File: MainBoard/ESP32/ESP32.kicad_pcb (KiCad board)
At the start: 2 copper layers, 97.5 x 77 mm, 42 parts, among them J1 Ultrasonic_1, J10 OUT1, J11 OUT1, J12 OUT1, J13 OUT1, J14 OUT1, J15 OUT1, J16 pH_SNS, J17 TDS_SNS, J18 Temp_SNS, J2 Ultrasonic_2, J3 Ultrasonic_3, J4 Barrel_Jack_Switch, J5 USB_B, J6 I2C_1, J7 I2C_1, J8 I2C_1, J9 SD_CARD_Module, Q1 2N7000, Q2 2N7000, Q3 2N7000, Q4 2N7000, Q5 2N7000, U1 ATtiny85-20PU, U2 LM296, U3 AMS1117-3.3, U4 ESP32-DevKit_V1

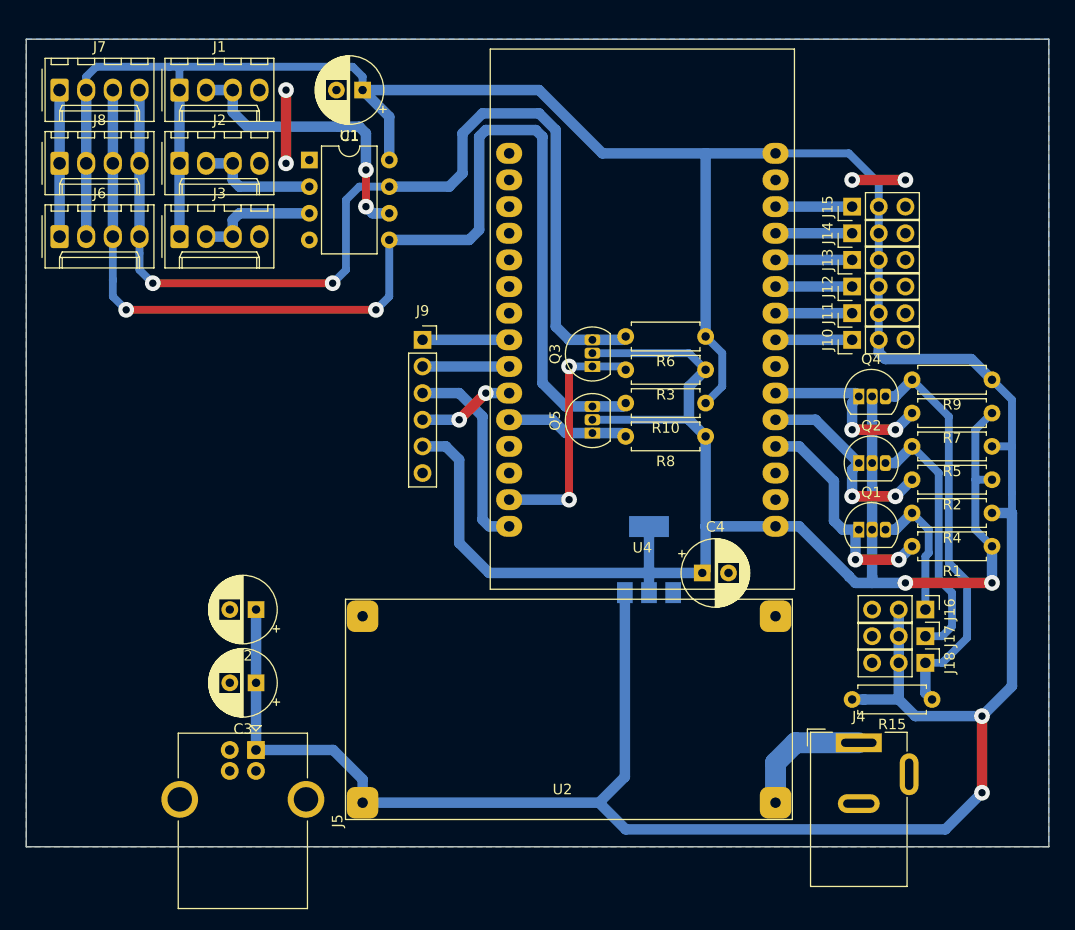
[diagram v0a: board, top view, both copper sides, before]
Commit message: Fix Main Board
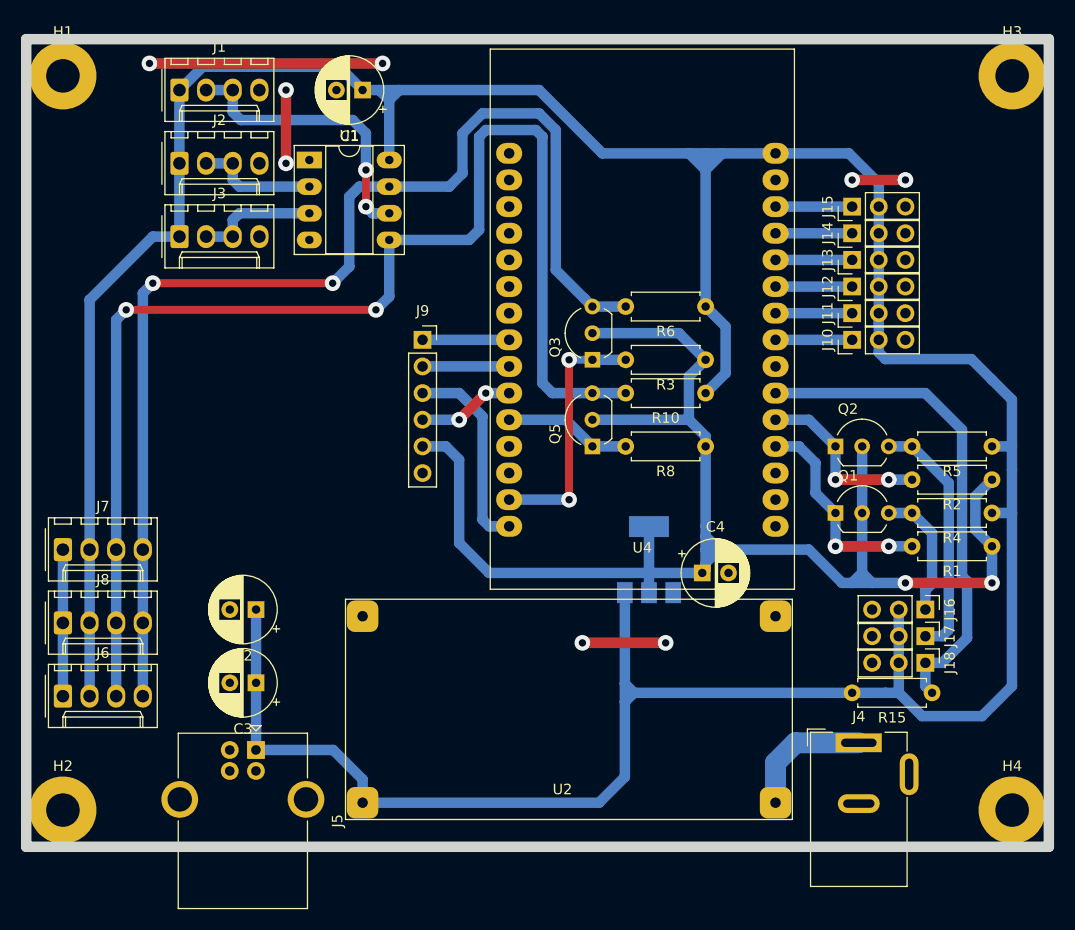
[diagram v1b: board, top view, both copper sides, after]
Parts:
- removed Q4: 2N7000, Package_TO_SOT_THT:TO-92L_Inline
- removed R7, R9: 10k, Resistor_THT:R_Axial_DIN0207_L6.3mm_D2.5mm_P7.62mm_Horizontal
- added H1: Mounting, MountingHole:MountingHole_3.2mm_M3_Pad, F.Cu at (107.0, 25.0)
- added H2: Mounting, MountingHole:MountingHole_3.2mm_M3_Pad, F.Cu at (107.0, 95.0)
- added H3: Mounting, MountingHole:MountingHole_3.2mm_M3_Pad, F.Cu at (197.5, 25.0)
- added H4: Mounting, MountingHole:MountingHole_3.2mm_M3_Pad, F.Cu at (197.5, 95.0)
- Q1, Q2, Q3, Q5: footprint Package_TO_SOT_THT:TO-92L_Inline -> Package_TO_SOT_THT:TO-92_Inline_Wide
- U1: footprint Package_DIP:DIP-8_W7.62mm -> Package_DIP:DIP-8_W7.62mm_Socket_LongPads
- moved J6 43.8 mm to (107.0, 84.1)
- moved J7 43.8 mm to (107.0, 70.2)
- moved J8 43.8 mm to (107.0, 77.2)
- moved R6 2.86 mm to (168.3, 47.0)
- moved Q1 2.73 mm to (180.7, 66.7)
- moved Q2 2.73 mm to (180.7, 60.3)
- moved Q5 1.27 mm to (157.5, 60.3)
- moved R10 0.95 mm to (168.3, 55.2)
- moved R3 0.95 mm to (168.3, 52.1)
- moved R8 0.95 mm to (168.3, 60.3)
- moved R15 0.64 mm to (189.9, 83.8)
- moved Q3 0.63 mm to (157.5, 52.1)
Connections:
- J18 pad 1: /H_TEMP_SNS -> /TEMP_SNS
- R15 pad 1: /H_TEMP_SNS -> /TEMP_SNS
- U4 pad 1: +3V3 -> Net-(U4-Pad1)
- U4 pad 6: /L_TEMP_SNS -> /TEMP_SNS
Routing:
- net /TEMP_SNS: track 0.00 -> 47.4 mm
- net /H_TEMP_SNS: track 38.7 -> 0.00 mm
- net GND: track 26.0 -> 56.2 mm, vias 4 -> 8
- net +5V: track 349.9 -> 379.0 mm, vias 2 -> 0
- net /L_TEMP_SNS: track 17.9 -> 0.00 mm, vias 2 -> 0
- net /H_SCL: track 96.9 -> 113.1 mm
- net /H_SDA: track 109.4 -> 124.5 mm
- net +3V3: track 150.5 -> 143.6 mm
- net /L_TDS_SNS: track 19.5 -> 17.2 mm
- net /L_pH_SNS: track 22.1 -> 20.5 mm
- net /H_TDS_SNS: track 24.9 -> 23.6 mm
- net /H_pH_SNS: track 13.2 -> 12.5 mm

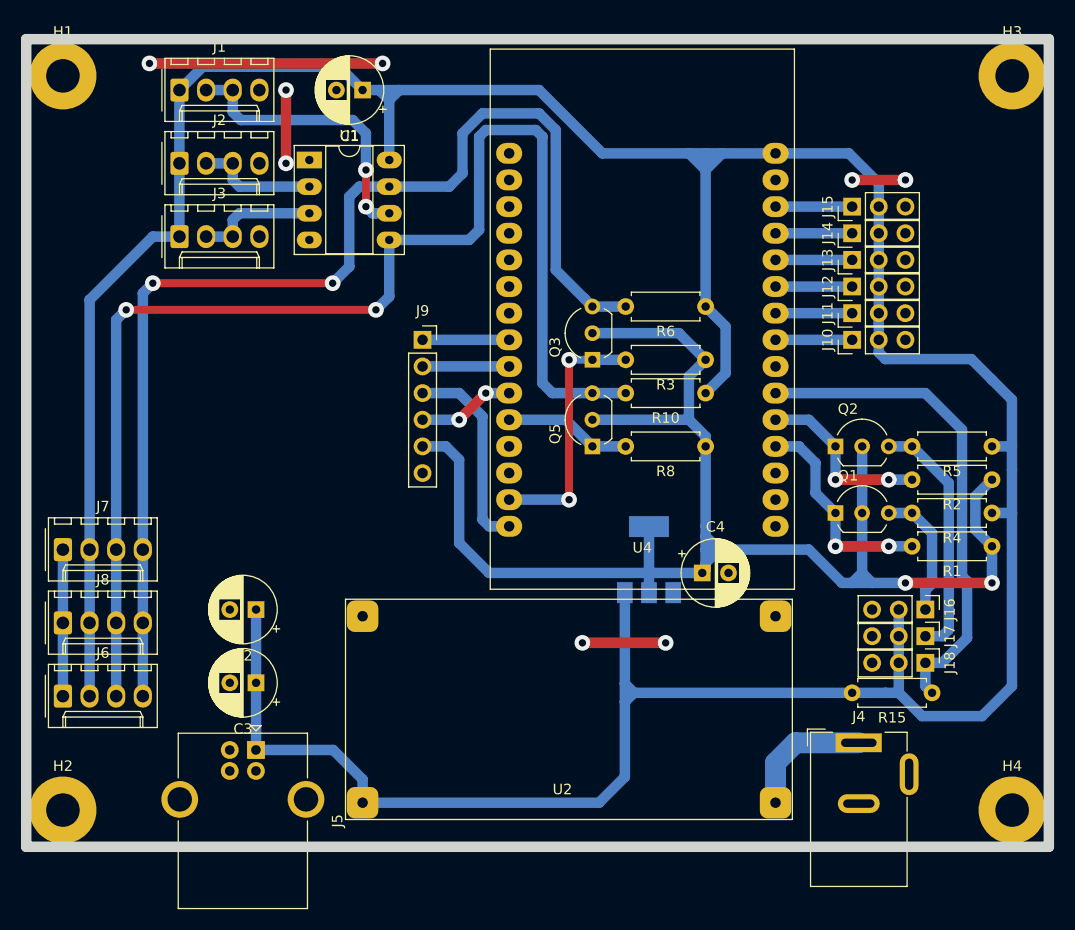
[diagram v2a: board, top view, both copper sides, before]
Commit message: Update Main Board
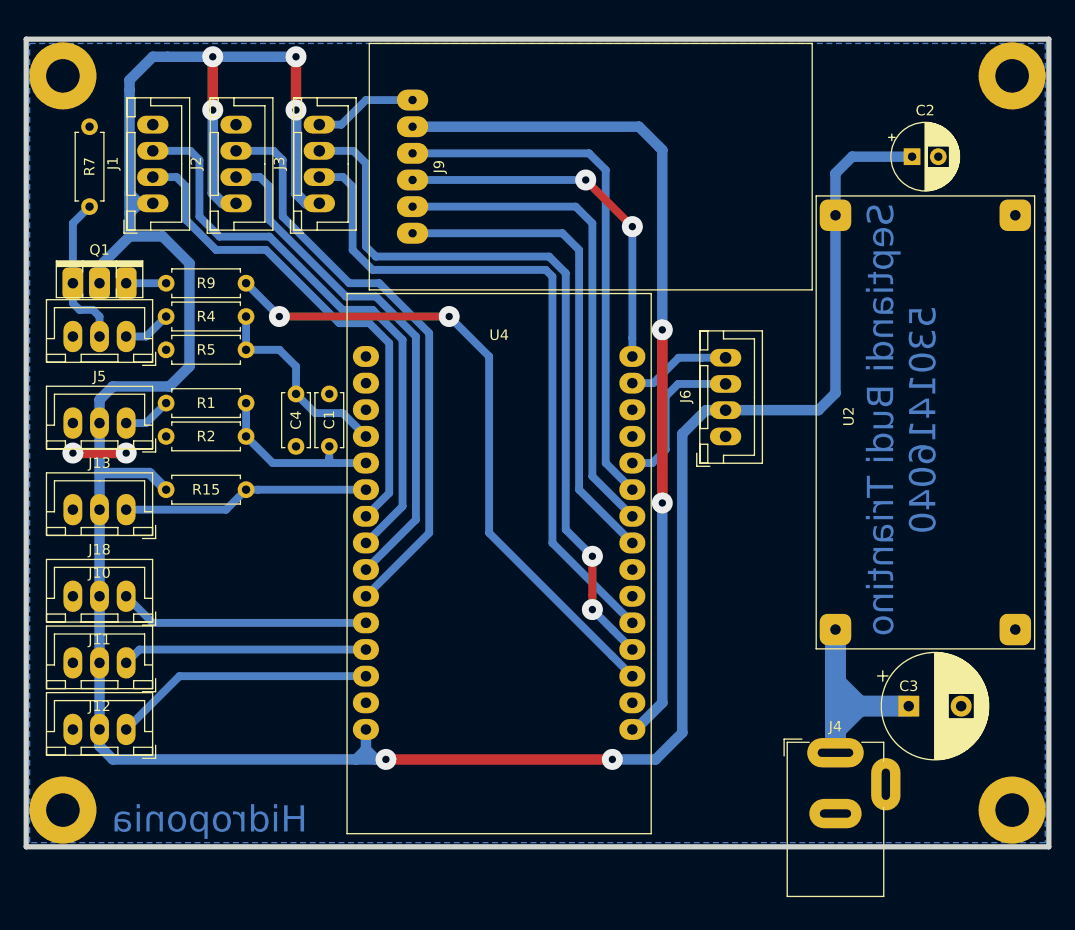
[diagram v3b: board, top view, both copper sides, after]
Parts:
- removed J14, J15: OUT1, Connector_PinHeader_2.54mm:PinHeader_1x03_P2.54mm_Vertical
- removed J16: pH_SNS, Connector_PinHeader_2.54mm:PinHeader_1x03_P2.54mm_Vertical
- removed J17: TDS_SNS, Connector_PinHeader_2.54mm:PinHeader_1x03_P2.54mm_Vertical
- removed J7, J8: I2C_1, Connector_Molex:Molex_KK-254_AE-6410-04A_1x04_P2.54mm_Vertical
- removed Q2, Q3, Q5: 2N7000, Package_TO_SOT_THT:TO-92_Inline_Wide
- removed R10, R3, R6, R8: 10k, Resistor_THT:R_Axial_DIN0207_L6.3mm_D2.5mm_P7.62mm_Horizontal
- removed U1: ATtiny85-20PU, Package_DIP:DIP-8_W7.62mm_Socket_LongPads
- removed U3: AMS1117-3.3, Package_TO_SOT_SMD:SOT-223-3_TabPin2
- added R7: 10k, Resistor_THT:R_Axial_DIN0207_L6.3mm_D2.5mm_P7.62mm_Horizontal, F.Cu at (109.5, 37.5)
- added R9: 200, Resistor_THT:R_Axial_DIN0207_L6.3mm_D2.5mm_P7.62mm_Horizontal, F.Cu at (124.5, 44.8)
- C1: value 10uf -> 104; footprint Capacitor_THT:CP_Radial_D6.3mm_P2.50mm -> Capacitor_THT:C_Disc_D5.0mm_W2.5mm_P5.00mm
- C3: value 47uf -> 1000u; footprint Capacitor_THT:CP_Radial_D6.3mm_P2.50mm -> Capacitor_THT:CP_Radial_D10.0mm_P5.00mm
- C4: value 47uf -> 104; footprint Capacitor_THT:CP_Radial_D6.3mm_P2.50mm -> Capacitor_THT:C_Disc_D5.0mm_W2.5mm_P5.00mm
- J1: value Ultrasonic_1 -> A MIX; footprint Connector_Molex:Molex_KK-254_AE-6410-04A_1x04_P2.54mm_Vertical -> DIY CONN:JST_XH_B4B-XH-A_1x04_P2.50_DIY
- J10, J18: footprint Connector_PinHeader_2.54mm:PinHeader_1x03_P2.54mm_Vertical -> DIY CONN:JST_XH_B3B-XH-A_1X03_P2.50mm_DIY
- J11: value OUT1 -> OUT2; footprint Connector_PinHeader_2.54mm:PinHeader_1x03_P2.54mm_Vertical -> DIY CONN:JST_XH_B3B-XH-A_1X03_P2.50mm_DIY
- J12: value OUT1 -> OUT3; footprint Connector_PinHeader_2.54mm:PinHeader_1x03_P2.54mm_Vertical -> DIY CONN:JST_XH_B3B-XH-A_1X03_P2.50mm_DIY
- J13: value OUT1 -> pH_SNS; footprint Connector_PinHeader_2.54mm:PinHeader_1x03_P2.54mm_Vertical -> DIY CONN:JST_XH_B3B-XH-A_1X03_P2.50mm_DIY
- J2: value Ultrasonic_2 -> B MIX; footprint Connector_Molex:Molex_KK-254_AE-6410-04A_1x04_P2.54mm_Vertical -> DIY CONN:JST_XH_B4B-XH-A_1x04_P2.50_DIY
- J3: value Ultrasonic_3 -> pH; footprint Connector_Molex:Molex_KK-254_AE-6410-04A_1x04_P2.54mm_Vertical -> DIY CONN:JST_XH_B4B-XH-A_1x04_P2.50_DIY
- J4: value Barrel_Jack_Switch -> Power Supply
- J5: value USB_B -> pH_SNS; footprint Connector_USB:USB_B_OST_USB-B1HSxx_Horizontal -> DIY CONN:JST_XH_B3B-XH-A_1X03_P2.50mm_DIY
- J6: footprint Connector_Molex:Molex_KK-254_AE-6410-04A_1x04_P2.54mm_Vertical -> DIY CONN:JST_XH_B4B-XH-A_1x04_P2.50_DIY
- J9: footprint Connector_PinSocket_2.54mm:PinSocket_1x06_P2.54mm_Vertical -> DIY:SD_Card
- Q1: value 2N7000 -> BD139; footprint Package_TO_SOT_THT:TO-92_Inline_Wide -> TO Package DIY:TO-126-3_DIY
- R1, R4: value 10k -> 5k1
- U2: value LM296 -> LM2596
- moved J12 81.1 mm to (113.0, 87.3), turned to 180 degrees
- moved R4 80.9 mm to (116.8, 47.9), turned to 0 degrees
- moved R1 79.9 mm to (116.8, 56.2), turned to 0 degrees
- moved J18 77.6 mm to (113.0, 66.4), turned to 180 degrees
- moved J11 76.8 mm to (113.0, 81.0), turned to 180 degrees
- moved C2 76.0 mm to (188.0, 32.7), turned to 0 degrees
- moved Q1 75.9 mm to (108.0, 44.8)
- moved J10 73.4 mm to (113.0, 74.6), turned to 180 degrees
- moved R5 71.7 mm to (124.5, 51.1)
- moved R2 71.2 mm to (124.5, 59.4)
- moved J13 70.9 mm to (113.0, 58.1), turned to 180 degrees
- moved R15 68.2 mm to (124.5, 64.5)
- moved J6 67.9 mm to (170.2, 59.4), turned to 90 degrees
- moved C3 62.3 mm to (187.6, 85.1), turned to 0 degrees
- moved C4 42.3 mm to (129.2, 55.3), turned to 270 degrees
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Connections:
- C1 pad 1: +5V -> /pH_SNS
- C3 pad 1: +5V -> +12V
- C4 pad 1: +3V3 -> /TDS_SNS
- J1 pad 2: /US_1 -> /A_TRIG
- J1 pad 3: /US_1 -> /A_ECHO
- J13 pad 1: /OUT4 -> Net-(J13-Pad1)
- J2 pad 2: /US_2 -> /B_TRIG
- J2 pad 3: /US_2 -> /B_ECHO
- J3 pad 2: /US_3 -> /pH_TRIG
- J3 pad 3: /US_3 -> /pH_ECHO
- J4 pad 1: Net-(J4-Pad1) -> +12V
- J5 pad 1: +5V -> Net-(J5-Pad1)
- J5 pad 3: Net-(J5-Pad3) -> GND
- J6 pad 3: /H_SDA -> /SDA
- J6 pad 4: /H_SCL -> /SCL
- Q1 pad 1: /L_pH_SNS -> Net-(J5-Pad2)
- Q1 pad 2: +3V3 -> +5V
- Q1 pad 3: /H_pH_SNS -> Net-(Q1-Pad3)
- R1 pad 1: +3V3 -> Net-(J13-Pad1)
- R1 pad 2: /L_pH_SNS -> /pH_SNS
- R2 pad 1: +3V3 -> /pH_SNS
- R2 pad 2: /L_TDS_SNS -> GND
- R4 pad 1: +5V -> Net-(J5-Pad1)
- R4 pad 2: /H_pH_SNS -> /TDS_SNS
- R5 pad 1: +5V -> /TDS_SNS
- R5 pad 2: /H_TDS_SNS -> GND
- U2 pad 1: Net-(J4-Pad1) -> +12V
- U4 pad 10: /OUT3 -> /B_ECHO
- U4 pad 11: /OUT4 -> /OUT1
- U4 pad 12: /OUT5 -> /OUT2
- U4 pad 13: /OUT6 -> /OUT3
- U4 pad 16: Net-(U4-Pad16) -> +3V3
- U4 pad 17: Net-(U4-Pad17) -> GND
- U4 pad 18: Net-(U4-Pad18) -> /TD_SW
- U4 pad 19: Net-(U4-Pad19) -> /pH_ECHO
- U4 pad 20: Net-(U4-Pad20) -> /pH_TRIG
- U4 pad 26: /L_SDA -> /SDA
- U4 pad 29: /L_SCL -> /SCL
- U4 pad 4: /L_pH_SNS -> /TDS_SNS
- U4 pad 5: /L_TDS_SNS -> /pH_SNS
- U4 pad 7: Net-(U4-Pad7) -> /A_TRIG
- U4 pad 8: /OUT1 -> /A_ECHO
- U4 pad 9: /OUT2 -> /B_TRIG
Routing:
- net /H_SDA: track 124.5 -> 0.00 mm, vias 2 -> 0
- net /H_SCL: track 113.1 -> 0.00 mm, vias 2 -> 0
- net /pH_ECHO: track 0.00 -> 71.5 mm, vias 0 -> 2
- net /pH_TRIG: track 0.00 -> 65.9 mm
- net +3V3: track 143.6 -> 81.3 mm
- net /TD_SW: track 0.00 -> 62.2 mm, vias 0 -> 2
- net +5V: track 379.0 -> 319.9 mm, vias 0 -> 6
- net /B_ECHO: track 0.00 -> 56.4 mm
- net /A_ECHO: track 0.00 -> 54.9 mm
- net /B_TRIG: track 0.00 -> 49.5 mm
- net /A_TRIG: track 0.00 -> 48.1 mm
- net /DAT0\MISO: track 9.31 -> 50.6 mm, vias 2 -> 0
- net GND: track 56.2 -> 14.9 mm, vias 8 -> 2
- net /CLK\SCK: track 8.25 -> 47.3 mm
- net /DAT3\CS: track 8.25 -> 46.6 mm
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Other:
- board text added: "Hidroponia"
- board text added: "Septiandi Budi Triantino 5301416040"
